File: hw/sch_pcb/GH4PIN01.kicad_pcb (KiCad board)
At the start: 2 copper layers, 40.1 x 40.1 mm, 7 parts, among them J1 SM04B-GHS-TB, J2 SM04B-GHS-TB, J3 HEADER_2x05_PARALLEL, M1 HOLE M3, M2 HOLE M3, M3 HOLE, M4 HOLE

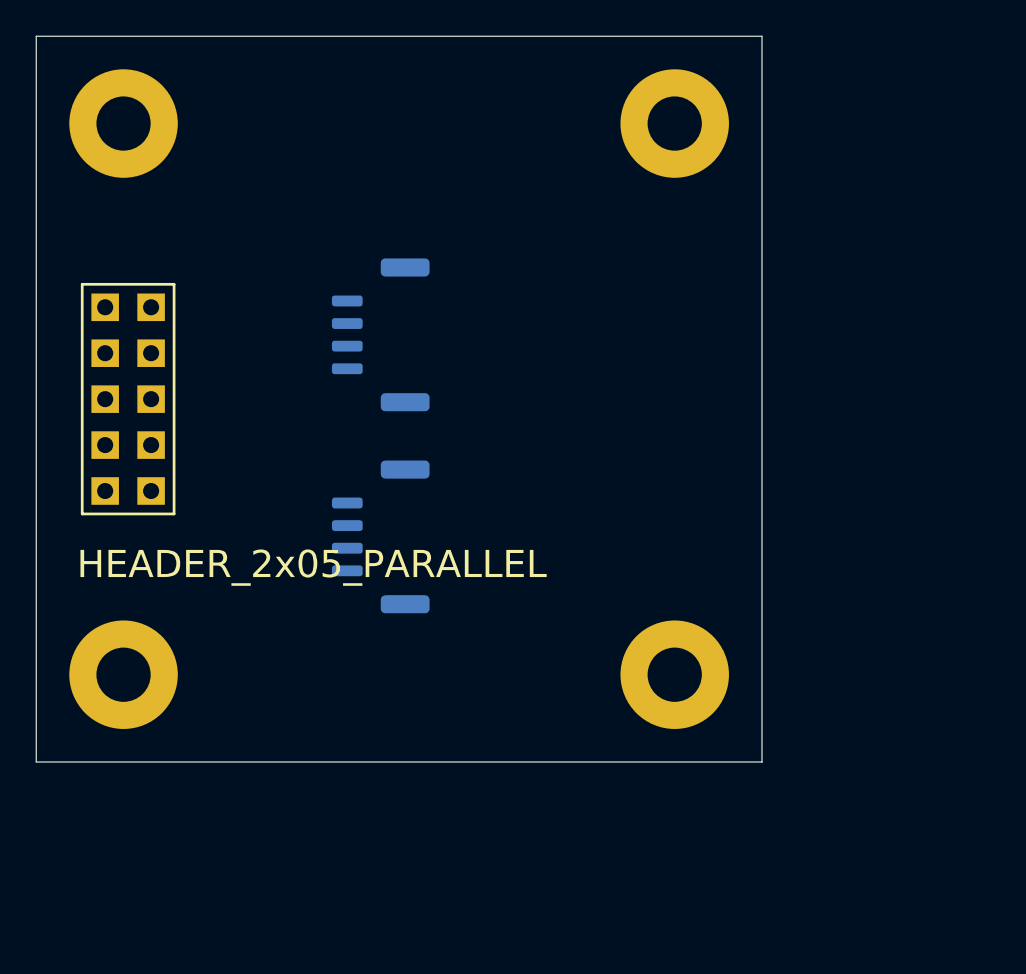
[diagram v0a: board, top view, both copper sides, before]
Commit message: The routed layout.
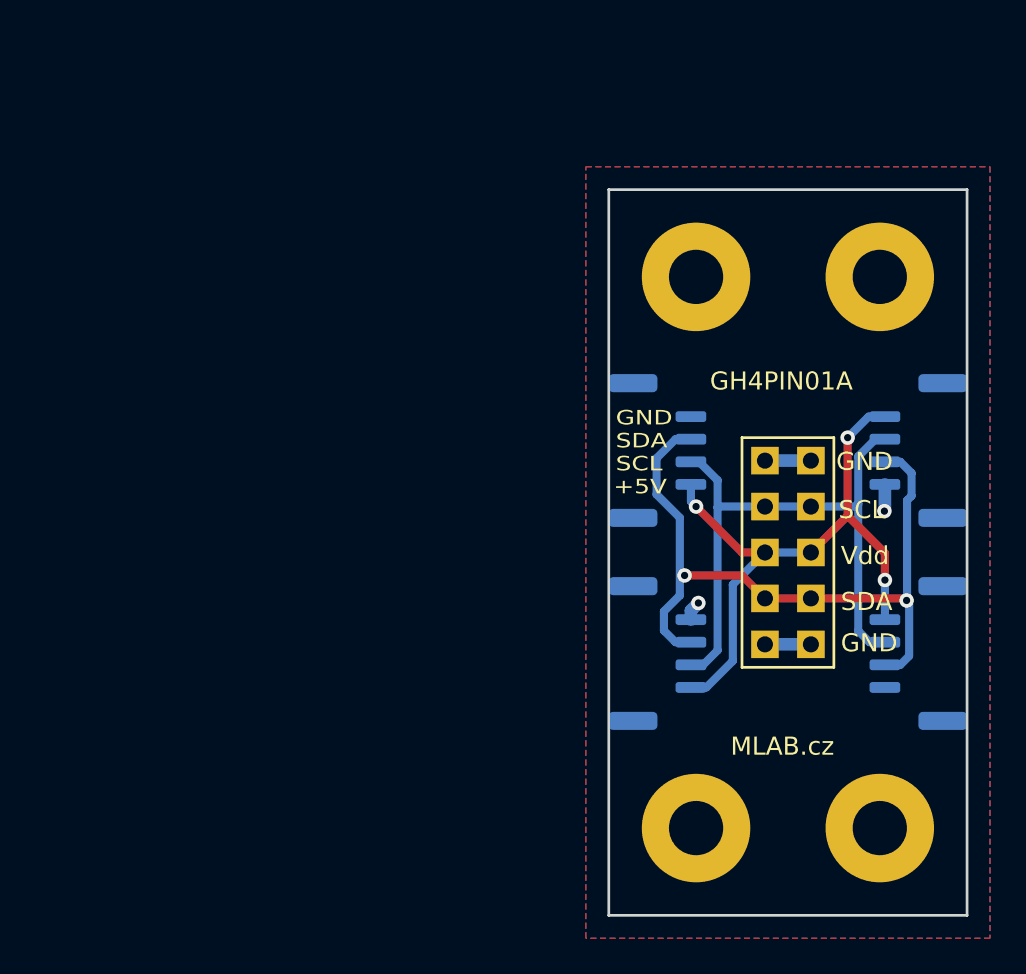
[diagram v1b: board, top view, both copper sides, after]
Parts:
- added J4: SM04B-GHS-TB, Connector_JST:JST_GH_SM04B-GHS-TB_1x04-1MP_P1.25mm_Horizontal, B.Cu at (141.3, 99.4)
- added J5: SM04B-GHS-TB, Connector_JST:JST_GH_SM04B-GHS-TB_1x04-1MP_P1.25mm_Horizontal, B.Cu at (141.3, 110.6)
- moved M2 42.7 mm to (153.6, 89.8)
- moved J3 37.5 mm to (148.5, 105.0)
- moved M3 32.8 mm to (143.4, 120.2)
- moved J1 30.4 mm to (155.7, 110.6)
- moved J2 30.4 mm to (155.7, 99.4)
- moved M4 14.2 mm to (153.6, 120.2)
- moved M1 8.56 mm to (143.4, 89.8)
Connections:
- net Net-(J2-Pad1) renamed /+5V
- net Net-(J3-Pad3) renamed /SCL
- net Net-(J3-Pad7) renamed /SDA
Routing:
- net /SDA: track 0.00 -> 40.9 mm, vias 0 -> 2
- net /+5V: track 0.00 -> 34.7 mm, vias 0 -> 3
- net /SCL: track 0.00 -> 34.2 mm
- net GND: track 0.00 -> 7.66 mm, vias 0 -> 2
- added copper zone on B.Cu, net GND
- added copper zone on F.Cu, net GND
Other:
- board size 40.1 x 40.1 mm -> 19.8 x 40.1 mm
- rule pad_to_mask_clearance: 0 -> 0.08
- board text added: "+5V"
- board text added: "GH4PIN01A"
- board text added: "GND"
- board text added: "MLAB.cz"
- board text added: "SCL"
- board text added: "SDA"
- board text added: "Vdd"
